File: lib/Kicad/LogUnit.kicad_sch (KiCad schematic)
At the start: 8 parts, among them U1 ProS3, U3 RFID-RC522

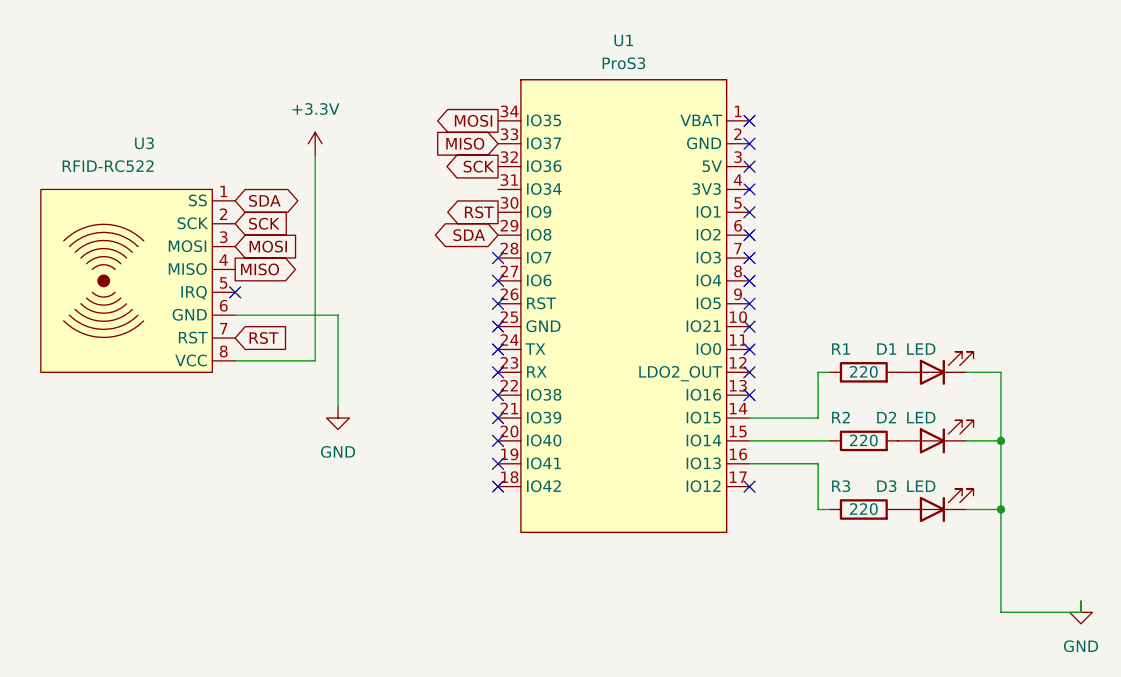
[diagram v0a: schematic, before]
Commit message: updated kicad
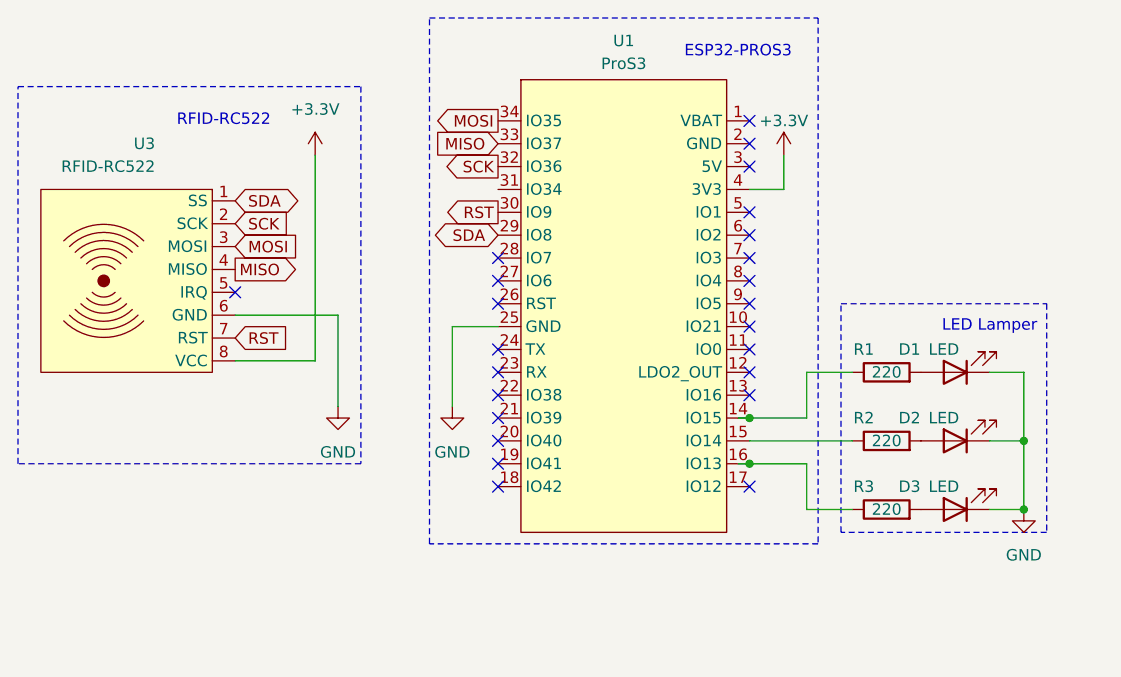
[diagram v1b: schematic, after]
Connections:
- net +3.3V: now also U1.4 (3V3)
- net GND: now also U1.25 (GND)
- no-connect marks 26 -> 24
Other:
- note added: "ESP32-PROS3"
- note added: "LED Lamper"
- note added: "RFID-RC522"
- moved on the sheet: D1, D2, D3, R1, R2, R3
